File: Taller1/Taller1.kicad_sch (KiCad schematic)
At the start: 9 parts, among them U1 DHT11, U2 Sensor de luz, U3 HL-69, U4 SX1262-XIAO

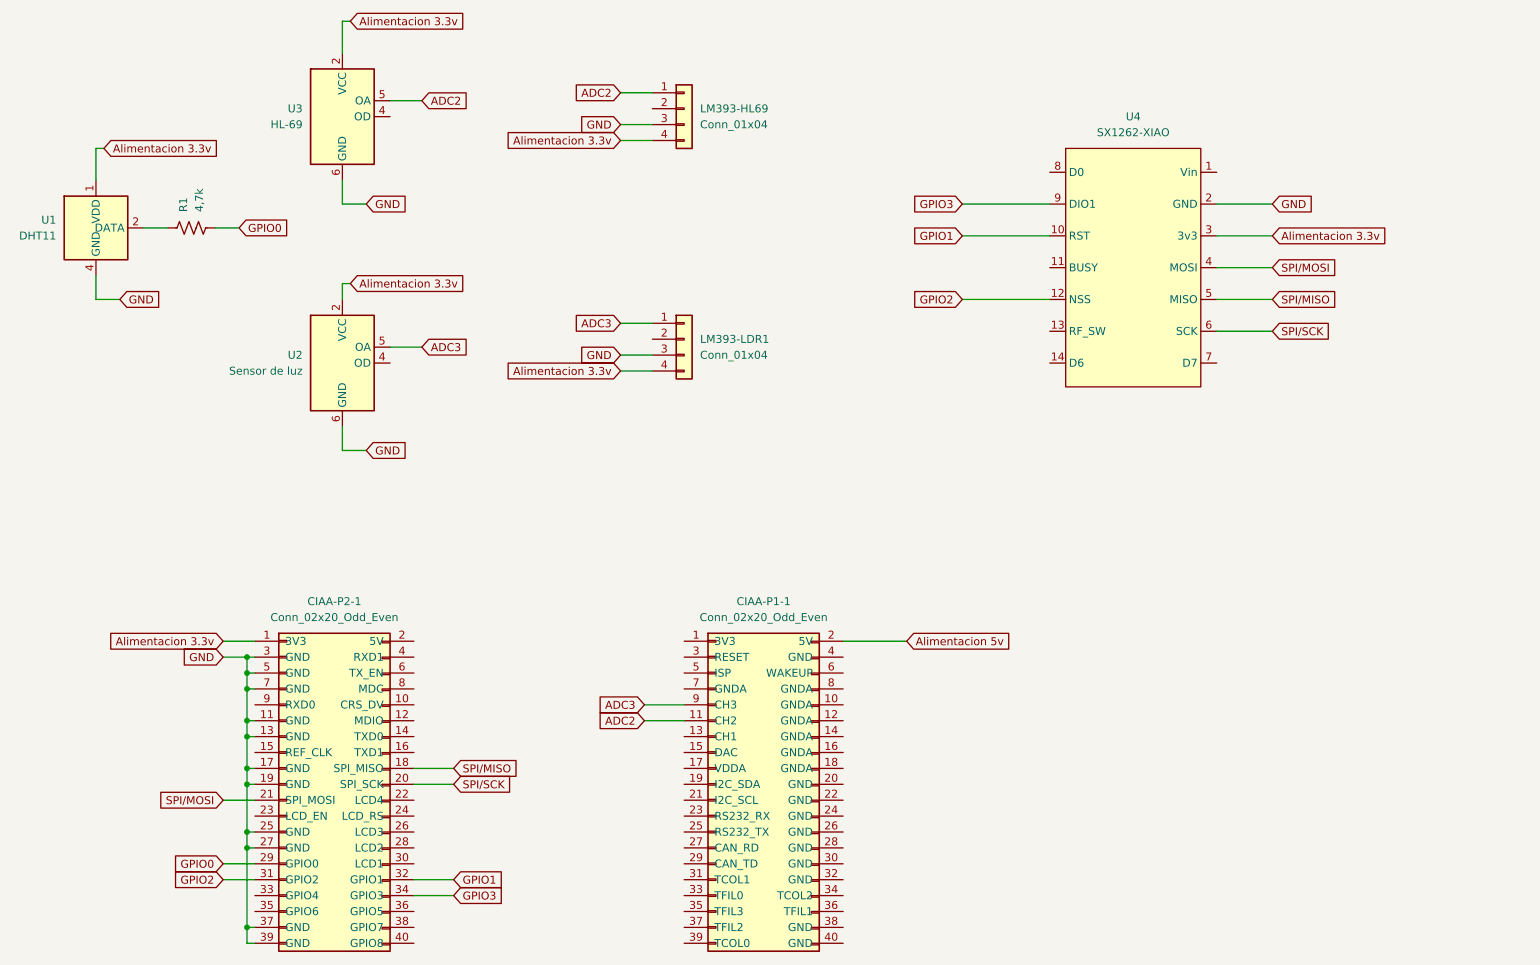
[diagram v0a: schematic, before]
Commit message: Ultima versao de KiCad
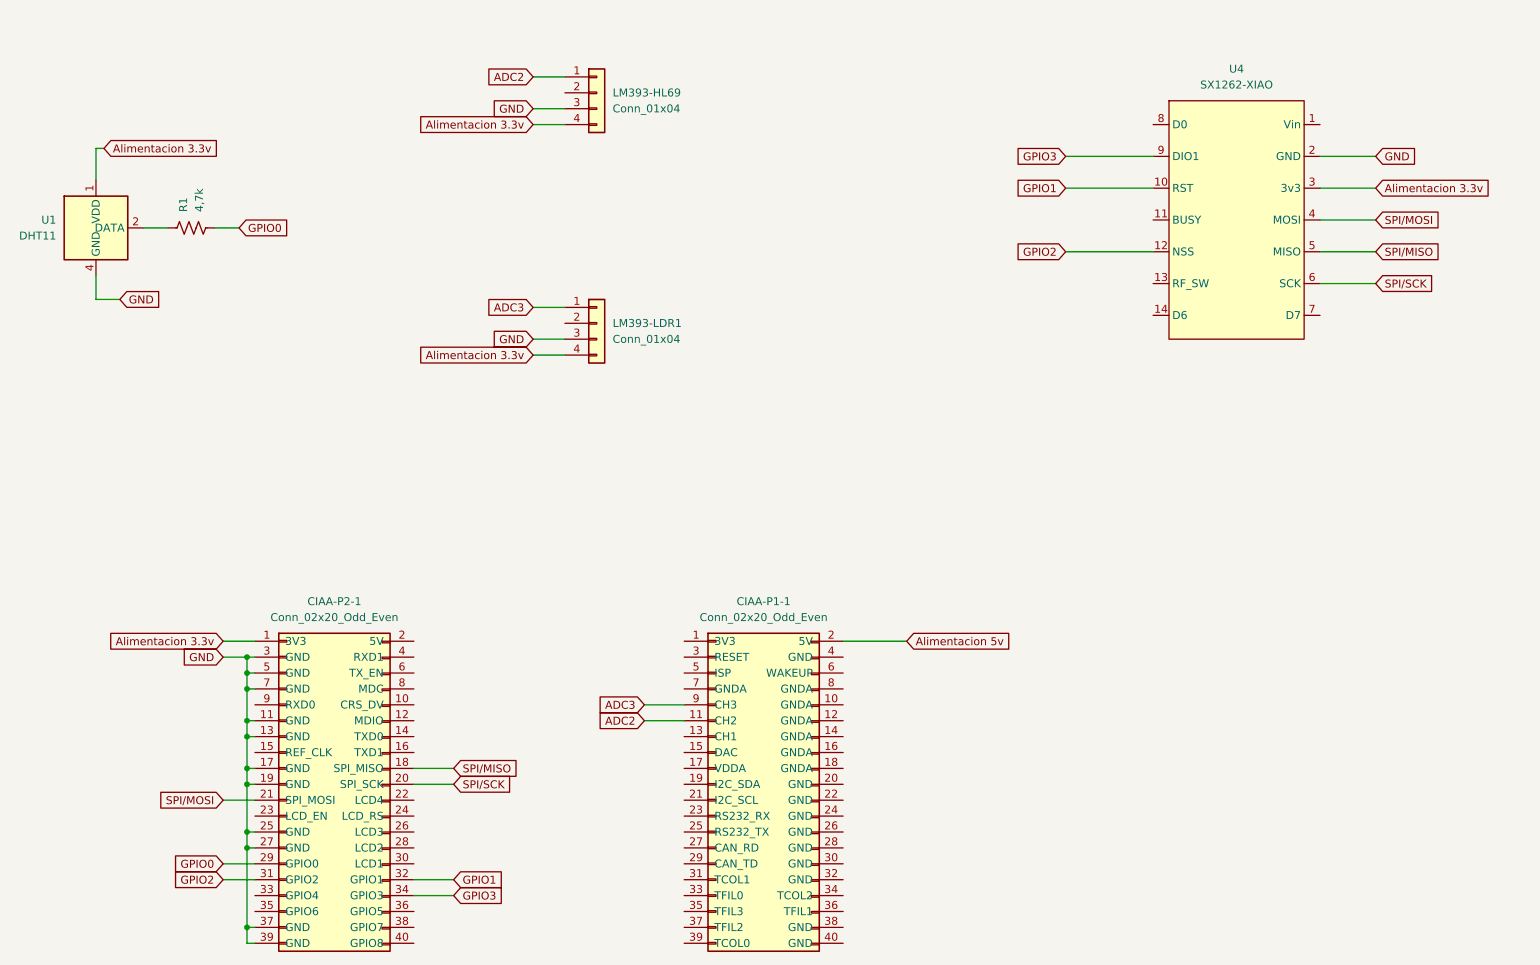
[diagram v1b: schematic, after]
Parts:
- removed U2: Sensor de luz, Sensor_Pressure:CFSensor_XGZP6859D_7x7mm, symbol Sensor_Pressure:XGZP6859D
- removed U3: HL-69, Sensor_Pressure:CFSensor_XGZP6859D_7x7mm, symbol Sensor_Pressure:XGZP6859D
- LM393-HL69, LM393-LDR1: footprint (none) -> Connector_PinHeader_2.54mm:PinHeader_1x04_P2.54mm_Vertical
- R1: footprint (none) -> Resistor_SMD:R_0805_2012Metric
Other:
- moved on the sheet: LM393-HL69, LM393-LDR1, U4
